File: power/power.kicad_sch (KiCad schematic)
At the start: 15 parts, among them J1 Barrel_Jack_Switch, J10 Screw_Terminal_01x02, J11 Screw_Terminal_01x02, Q1 IRFZ44N, Q2 IRFZ44N, Q3 IRF9540N, U1 LTC4412xS6

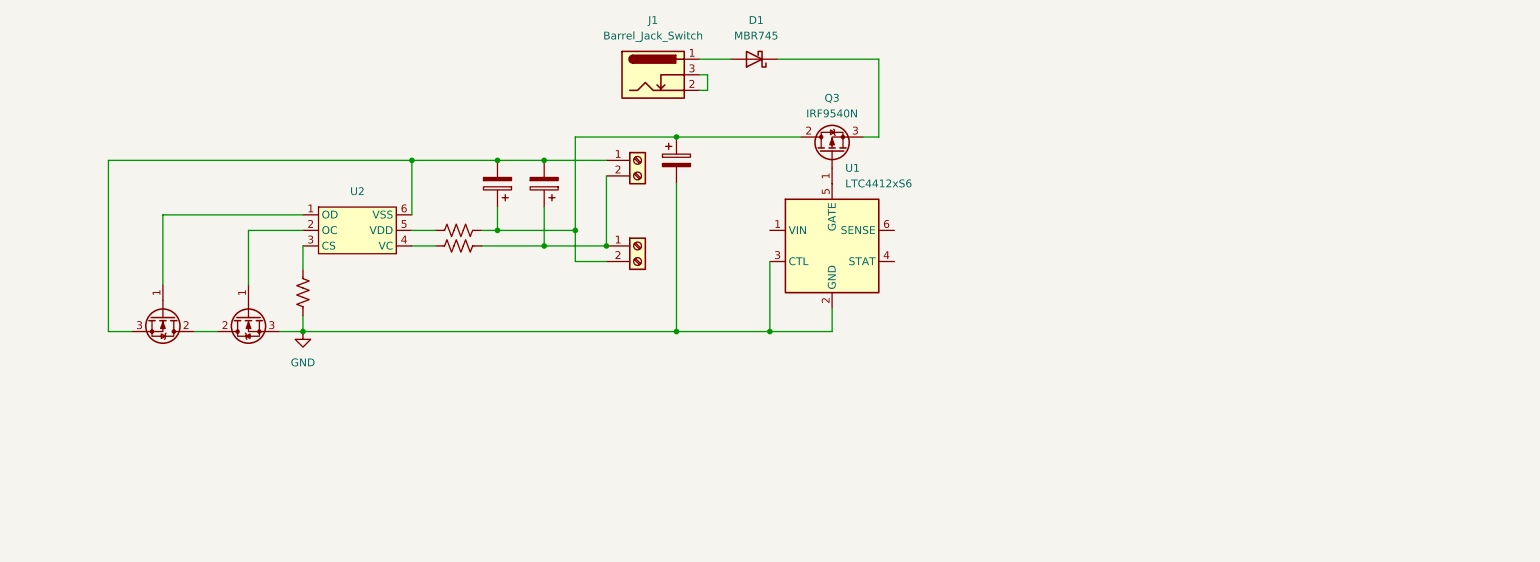
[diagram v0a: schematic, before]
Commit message: refresh
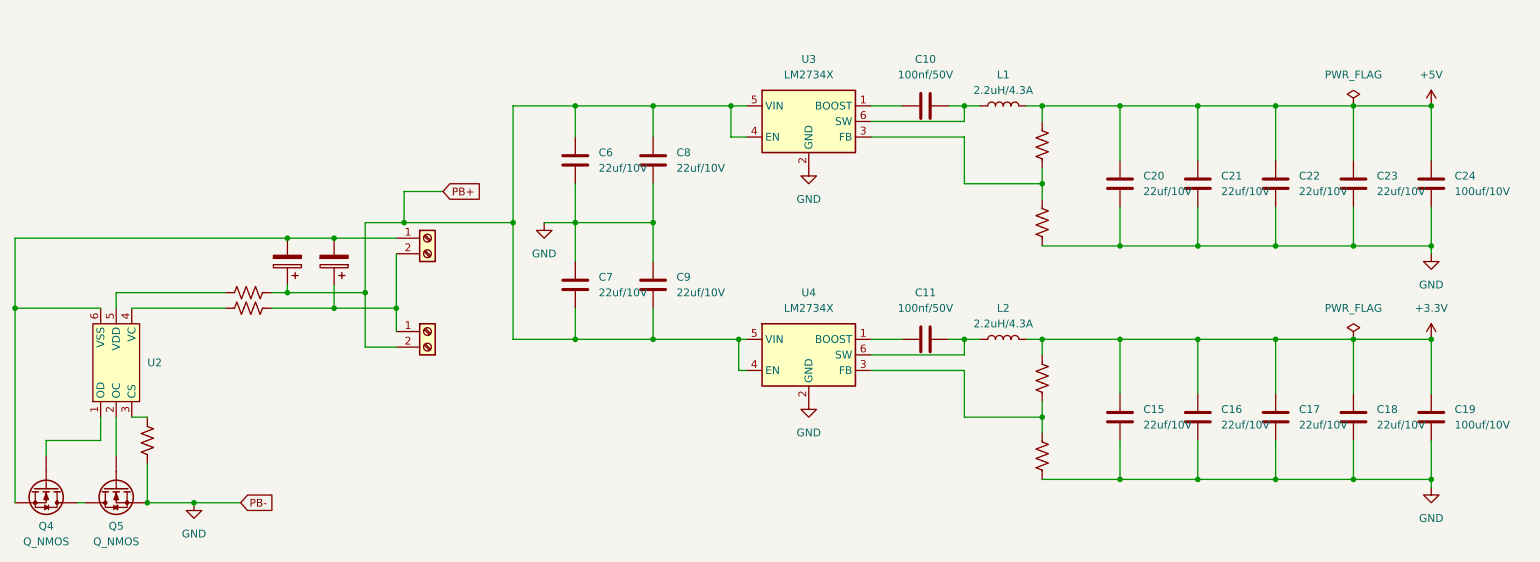
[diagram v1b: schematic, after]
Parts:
- removed C1, C2: C_Polarized, Capacitor_SMD:C_0805_2012Metric_Pad1.18x1.45mm_HandSolder, symbol Device:C_Polarized
- removed C3: 10u, Capacitor_SMD:C_0805_2012Metric_Pad1.18x1.45mm_HandSolder, symbol Device:C_Polarized
- removed D1: MBR745, Package_TO_SOT_THT:TO-220-2_Vertical, symbol Diode:MBR745
- removed J1: Barrel_Jack_Switch, symbol Connector:Barrel_Jack_Switch
- removed J10, J11: Screw_Terminal_01x02, Connector_JST:JST_EH_B2B-EH-A_1x02_P2.50mm_Vertical, symbol Connector:Screw_Terminal_01x02
- removed Q1, Q2: IRFZ44N, Package_TO_SOT_THT:TO-220-3_Vertical, symbol Transistor_FET:BUZ11
- removed Q3: IRF9540N, Package_TO_SOT_THT:TO-220-3_Vertical, symbol Transistor_FET:IRF9540N
- removed R1, R2, R3: R_US, Resistor_SMD:R_0805_2012Metric_Pad1.20x1.40mm_HandSolder, symbol Device:R_US
- removed U1: LTC4412xS6, Package_TO_SOT_SMD:TSOT-23-6, symbol Power_Management:LTC4412xS6
- added C10, C11: 100nf/50V, Capacitor_SMD:C_0402_1005Metric_Pad0.74x0.62mm_HandSolder, symbol Device:C
- added C15, C16, C17, C18, C20, C21, C22, C23, C6, C7, C8, C9: 22uf/10V, A_HDJ_Library:C_0603_1608Metric, symbol Device:C
- added C19, C24: 100uf/10V, A_HDJ_Library:C_0603_1608Metric, symbol Device:C
- added C4, C5: C_Polarized, Capacitor_SMD:C_0805_2012Metric_Pad1.18x1.45mm_HandSolder, symbol Device:C_Polarized
- added J12, J13: Screw_Terminal_01x02, Connector_JST:JST_EH_B2B-EH-A_1x02_P2.50mm_Vertical, symbol Connector:Screw_Terminal_01x02
- added L1, L2: 2.2uH/4.3A, Inductor_THT:L_Toroid_Vertical_L10.0mm_W5.0mm_P5.08mm, symbol Device:L
- added Q4, Q5: Q_NMOS, Package_TO_SOT_THT:TO-247-3_Horizontal_TabDown, symbol Device:Q_NMOS
- added R10, R4, R5, R6, R7, R8, R9: R_US, Resistor_SMD:R_0805_2012Metric_Pad1.20x1.40mm_HandSolder, symbol Device:R_US
- added U3, U4: LM2734X, Package_TO_SOT_SMD:TSOT-23-6, symbol Regulator_Switching:LM2734X
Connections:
- net GND: now also C15.1, C16.1, C17.1, C18.1, C19.1, C20.1, C21.1, C22.1, C23.1, C24.1, C6.2, C7.1, C8.2, C9.1, Q5.S, R10.1, R6.1, R8.1, U3.2 (GND), U4.2 (GND)
- net at U2.2 (OC): now also Q5.G
- net at U2.5 (VDD): now also R4.1
- net at U2.6 (VSS): now also C4.2, C5.2, J12.1 (Pin_1), Q4.S
- net at U2.1 (OD): now also Q4.G
- net at U2.3 (CS): now also R6.2
- net at U2.4 (VC): now also R5.1
- new net: C5.1, J12.2 (Pin_2), J13.1 (Pin_1), R5.2
- new net: C10.1, U3.1 (BOOST)
- new net: R7.1, R8.2, U3.3 (FB)
- new net: C10.2, L1.1, U3.6 (SW)
- new net: C11.2, L2.1, U4.6 (SW)
- new net: C11.1, U4.1 (BOOST)
- new net: R10.2, R9.1, U4.3 (FB)
- new net: Q4.D, Q5.D
- new net +3.3V: C15.2, C16.2, C17.2, C18.2, C19.2, L2.2, R9.2
- new net +5V: C20.2, C21.2, C22.2, C23.2, C24.2, L1.2, R7.2
- new net PB+: C4.1, C6.1, C7.2, C8.1, C9.2, J13.2 (Pin_2), R4.2, U3.4 (EN), U3.5 (VIN), U4.4 (EN), U4.5 (VIN)
